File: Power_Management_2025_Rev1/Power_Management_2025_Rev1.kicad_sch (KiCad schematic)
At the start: 103 parts, among them J1 RJ45_LED_Shielded, Q1 BSS138, Q2 IPB180N10S4-02, Q3 IPB180N10S4-02, U1 Teensy4.1_DEV-16771, U10 LT1910, U11 LT1910, U12 PKE3316ZPI, U13 PKE3316ZPI, U2 OKI-78SR-3.3_1.5-W36-C, U3 ACS756xCB-050B-PFF, U4 ${SIM.PARAMS}, U5 ${SIM.PARAMS}, U6 ${SIM.PARAMS}, U7 ${SIM.PARAMS}, U8 ${SIM.PARAMS}, U9 ${SIM.PARAMS}

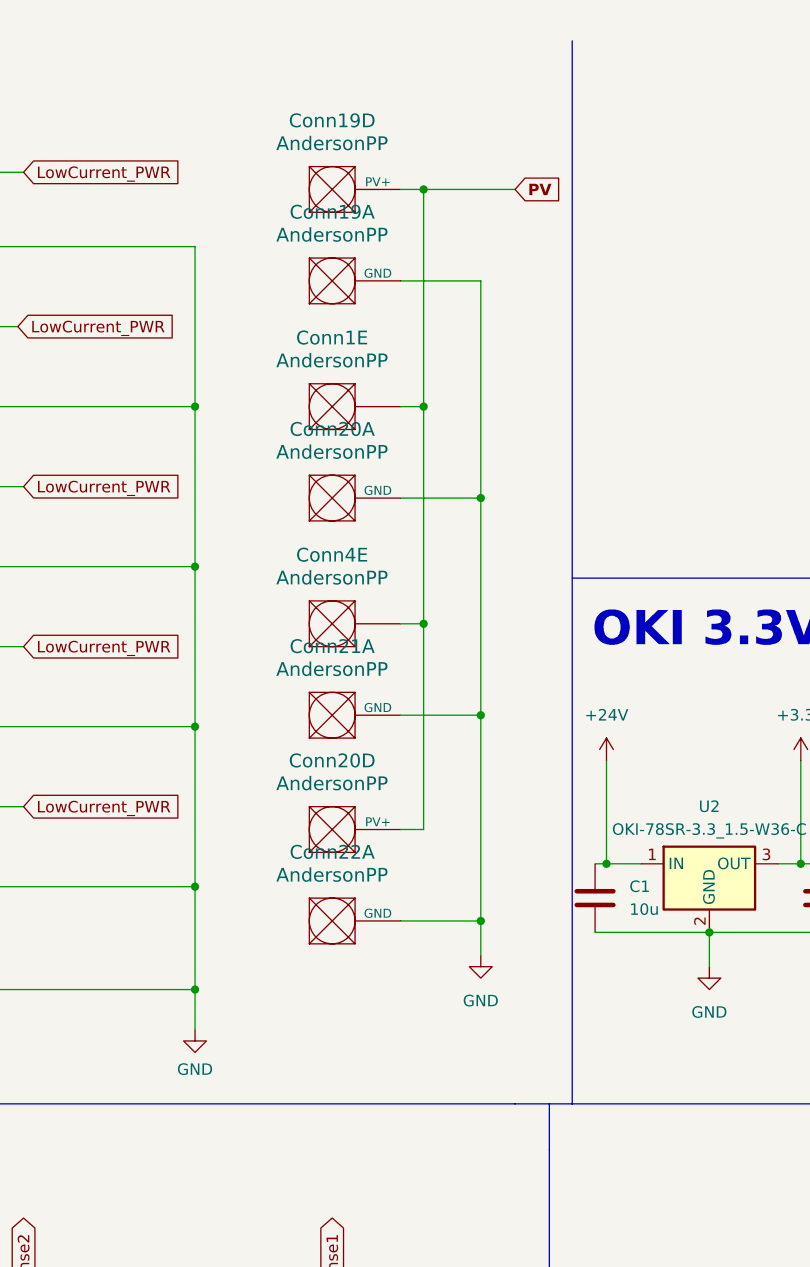
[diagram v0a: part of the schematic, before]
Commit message: Added set of andersons
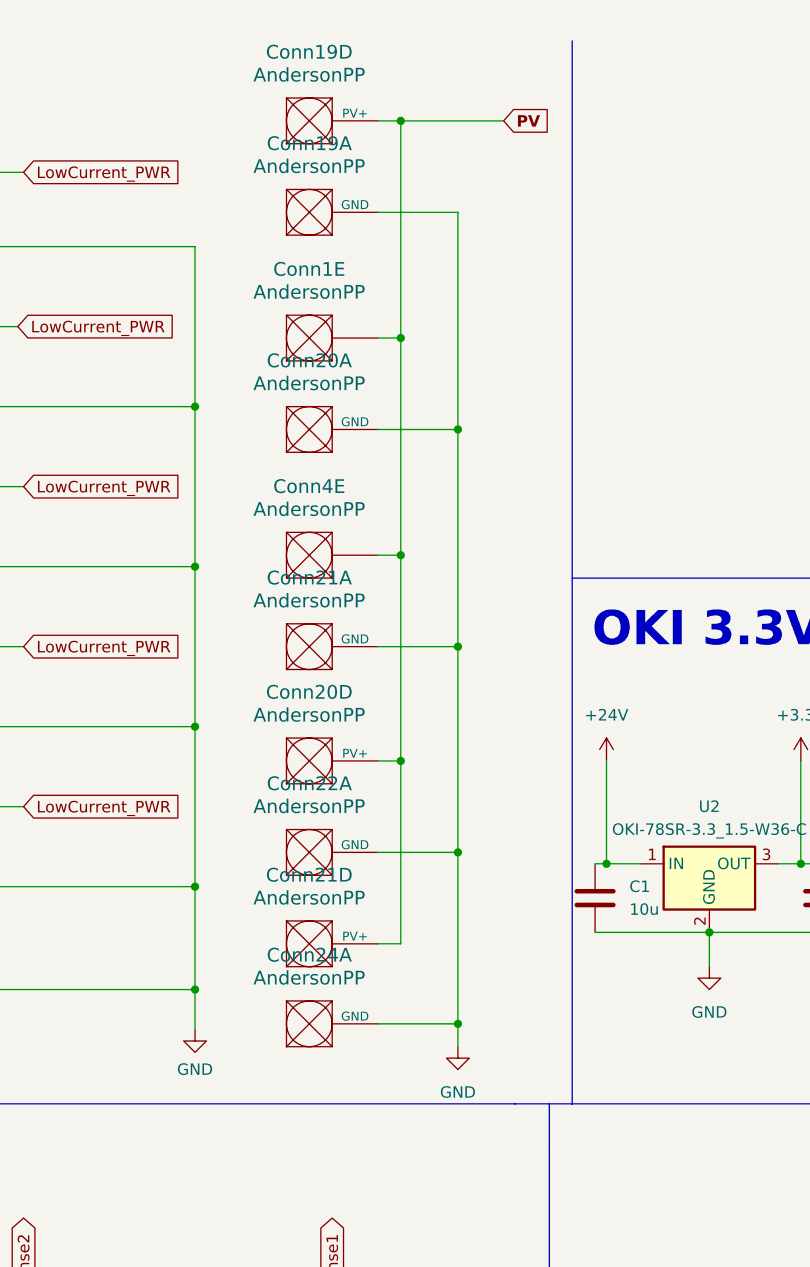
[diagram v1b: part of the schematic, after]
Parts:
- added unit 4 of Conn21
- added Conn24: AndersonPP, symbol MRDT_Connectors:AndersonPP
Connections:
- net GND: now also Conn24.1 (GND)
- net PV: now also Conn21.4 (PV+)
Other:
- moved on the sheet: Conn19A, Conn19D, Conn1E, Conn20A, Conn20D, Conn21A, Conn22A, Conn4E
